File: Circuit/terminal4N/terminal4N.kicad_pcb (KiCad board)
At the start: 2 copper layers, 10 parts, among them J1 Conn_01x05_Male, J2 Conn_02x08_Odd_Even, J3 Conn_01x02_Male, U1 4051

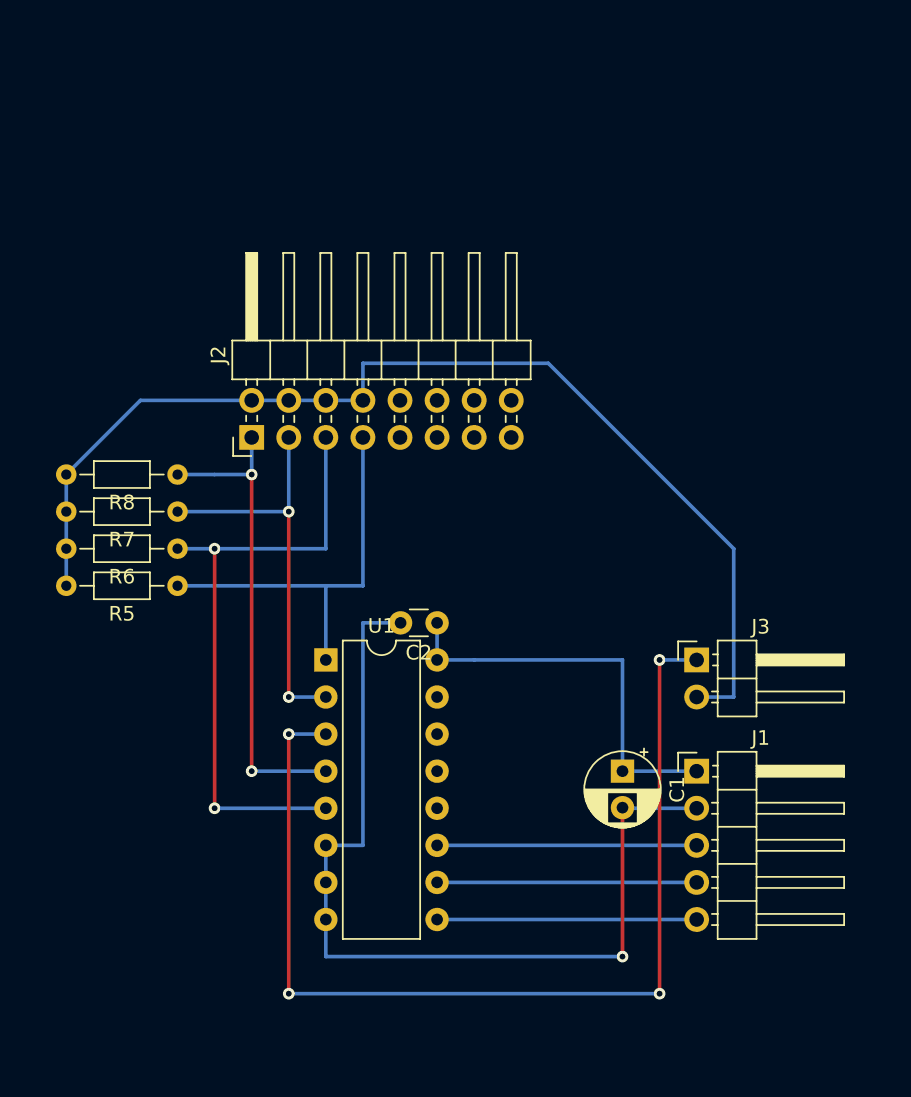
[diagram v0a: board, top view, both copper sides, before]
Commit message: ECM対策
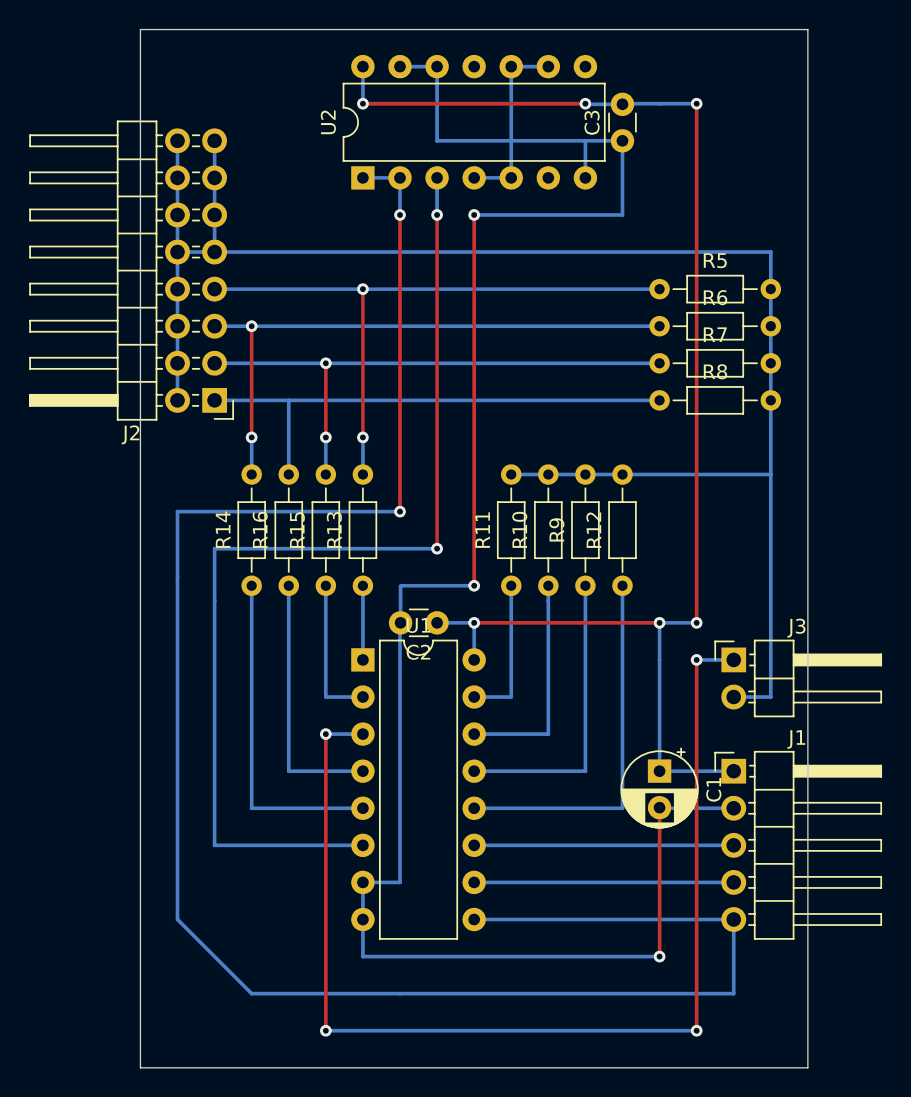
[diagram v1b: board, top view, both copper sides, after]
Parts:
- added C3: 0.1u, Capacitor_THT:C_Disc_D3.0mm_W1.6mm_P2.50mm, F.Cu at (137.2, 40.6)
- added R10: 220, Resistor_THT:R_Axial_DIN0204_L3.6mm_D1.6mm_P7.62mm_Horizontal, F.Cu at (132.1, 71.1)
- added R11: 220, Resistor_THT:R_Axial_DIN0204_L3.6mm_D1.6mm_P7.62mm_Horizontal, F.Cu at (129.5, 71.1)
- added R12: 220, Resistor_THT:R_Axial_DIN0204_L3.6mm_D1.6mm_P7.62mm_Horizontal, F.Cu at (137.2, 71.1)
- added R13: 220, Resistor_THT:R_Axial_DIN0204_L3.6mm_D1.6mm_P7.62mm_Horizontal, F.Cu at (119.4, 71.1)
- added R14: 220, Resistor_THT:R_Axial_DIN0204_L3.6mm_D1.6mm_P7.62mm_Horizontal, F.Cu at (111.8, 71.1)
- added R15: 220, Resistor_THT:R_Axial_DIN0204_L3.6mm_D1.6mm_P7.62mm_Horizontal, F.Cu at (116.8, 71.1)
- added R16: 220, Resistor_THT:R_Axial_DIN0204_L3.6mm_D1.6mm_P7.62mm_Horizontal, F.Cu at (114.3, 71.1)
- added R9: 220, Resistor_THT:R_Axial_DIN0204_L3.6mm_D1.6mm_P7.62mm_Horizontal, F.Cu at (134.6, 71.1)
- added U2: 74HC00, Package_DIP:DIP-14_W7.62mm, F.Cu at (119.4, 43.2)
- moved R5 38.8 mm to (139.7, 50.8), turned to 0 degrees
- moved R6 36.4 mm to (139.7, 53.3), turned to 0 degrees
- moved R7 34.5 mm to (139.7, 55.9), turned to 0 degrees
- moved R8 33.4 mm to (139.7, 58.4), turned to 0 degrees
- moved J2 3.59 mm to (109.2, 58.4), turned to 180 degrees
- moved C1 2.54 mm to (139.7, 83.8)
- moved J1 2.54 mm to (144.8, 83.8)
- moved J3 2.54 mm to (144.8, 76.2)
- moved U1 2.54 mm to (119.4, 76.2)
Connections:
- J2 pad 10: (no net) -> Net-(J2-Pad10)
- J2 pad 11: (no net) -> Net-(J2-Pad10)
- J2 pad 12: (no net) -> Net-(J2-Pad10)
- J2 pad 13: (no net) -> Net-(J2-Pad10)
- J2 pad 14: (no net) -> Net-(J2-Pad10)
- J2 pad 15: (no net) -> Net-(J2-Pad10)
- J2 pad 16: (no net) -> Net-(J2-Pad10)
- J2 pad 2: Net-(J2-Pad2) -> Net-(J2-Pad10)
- J2 pad 4: Net-(J2-Pad2) -> Net-(J2-Pad10)
- J2 pad 6: Net-(J2-Pad2) -> Net-(J2-Pad10)
- J2 pad 8: Net-(J2-Pad2) -> Net-(J2-Pad10)
- J2 pad 9: (no net) -> Net-(J2-Pad10)
- J3 pad 2: Net-(J2-Pad2) -> Net-(J2-Pad10)
- R5 pad 2: Net-(J2-Pad2) -> Net-(J2-Pad10)
- R6 pad 2: Net-(J2-Pad2) -> Net-(J2-Pad10)
- R7 pad 2: Net-(J2-Pad2) -> Net-(J2-Pad10)
- R8 pad 2: Net-(J2-Pad2) -> Net-(J2-Pad10)
- U1 pad 1: Net-(J2-Pad7) -> Net-(R13-Pad1)
- U1 pad 12: (no net) -> Net-(R12-Pad1)
- U1 pad 13: (no net) -> Net-(R9-Pad1)
- U1 pad 14: (no net) -> Net-(R10-Pad1)
- U1 pad 15: (no net) -> Net-(R11-Pad1)
- U1 pad 2: Net-(J2-Pad3) -> Net-(R15-Pad1)
- U1 pad 4: Net-(J2-Pad1) -> Net-(R16-Pad1)
- U1 pad 5: Net-(J2-Pad5) -> Net-(R14-Pad1)
- U1 pad 6: GND -> Net-(U1-Pad6)
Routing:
- net Net-(J2-Pad10): track 0.00 -> 116.8 mm
- net Net-(J1-Pad5): track 17.8 -> 131.6 mm, vias 0 -> 2
- net GND: track 63.6 -> 144.8 mm, vias 1 -> 3
- net Net-(J2-Pad2): track 75.9 -> 0.00 mm
- net Net-(U1-Pad6): track 0.00 -> 71.1 mm, vias 0 -> 2
- net VDD: track 27.9 -> 96.6 mm, vias 0 -> 6
- net Net-(R12-Pad1): track 0.00 -> 25.4 mm
- net Net-(R14-Pad1): track 0.00 -> 22.9 mm
- net Net-(R9-Pad1): track 0.00 -> 20.3 mm
- net Net-(R16-Pad1): track 0.00 -> 17.8 mm
- net Net-(R10-Pad1): track 0.00 -> 15.2 mm
- net Net-(J2-Pad7): track 27.9 -> 43.2 mm, vias 0 -> 2
- net Net-(J2-Pad3): track 27.9 -> 38.1 mm
- net Net-(R15-Pad1): track 0.00 -> 10.2 mm
- net Net-(R11-Pad1): track 0.00 -> 10.2 mm
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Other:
- board outline added: 45.7 x 71.1 mm
- board text added: "Akizuki Type C Board (17x27)"
